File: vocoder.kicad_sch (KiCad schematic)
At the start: 66 parts, among them J1 AudioJack4, J2 Conn_01x02_Socket, J3 Conn_01x02_Pin, J4 USB_C_Receptacle_USB2.0_16P, Q1 Q_NPN_BCE, Q2 Q_NPN_BCE, Q3 AO3401A, Q4 Q_NPN_BCE, SW1 SW_SPDT, SW2 SW_Push, SW3 SW_Push, U2 MAX98357A, U3 BQ24074RGT, U4 TPS63031DSK, U5 ADAU1761, U6 ${SIM.PARAMS}, U7 ESP32-S3-WROOM-1

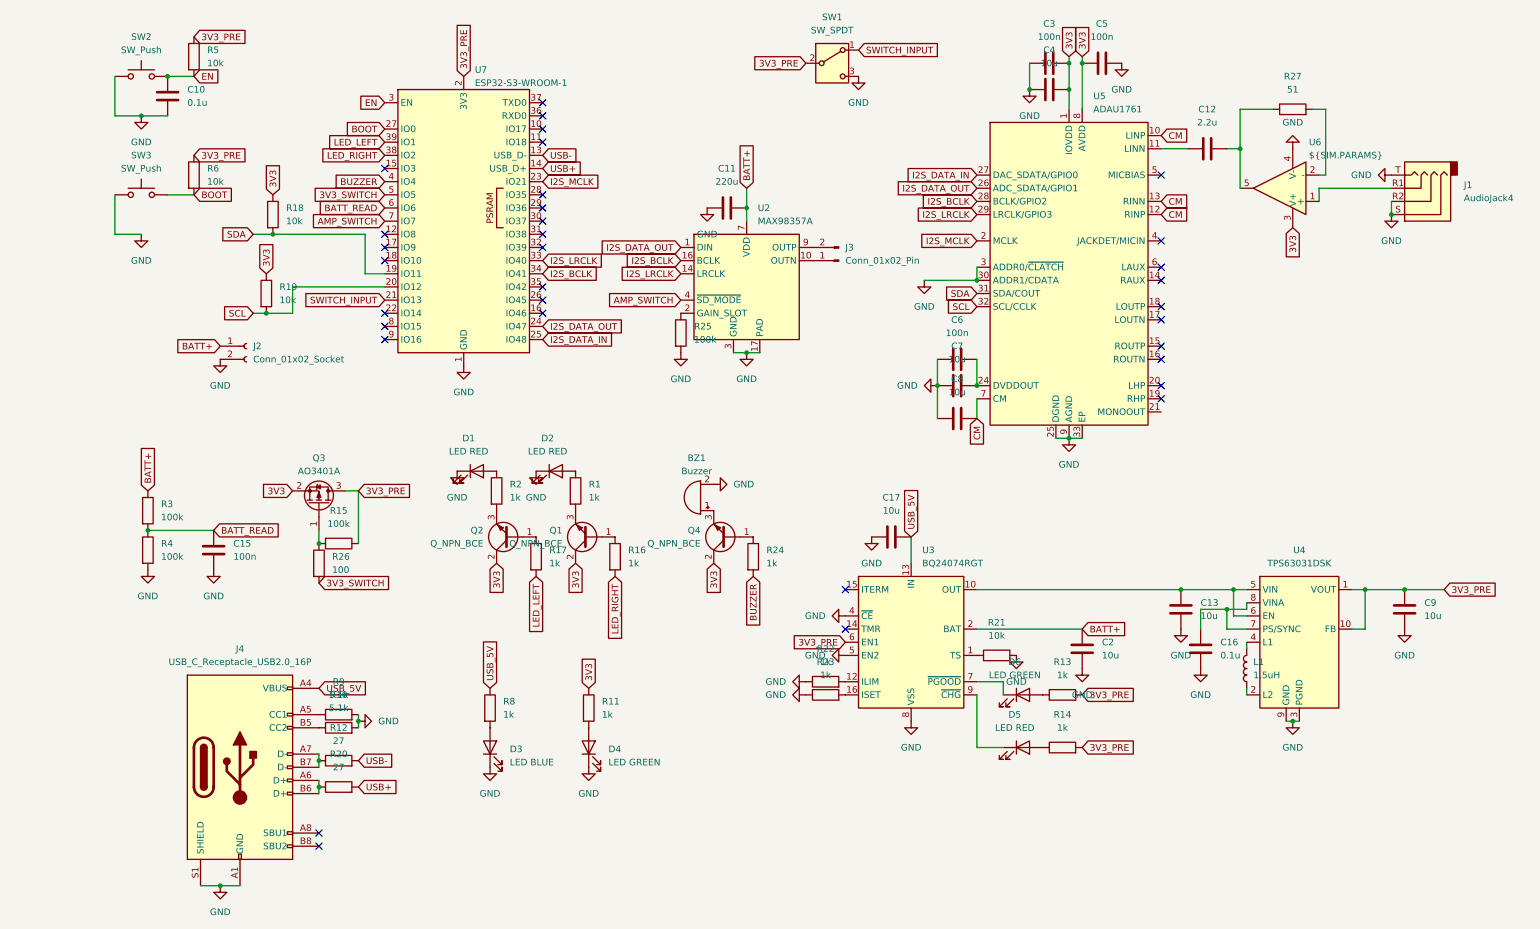
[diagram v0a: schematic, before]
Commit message: semi working before removing battery and adding necessary changes
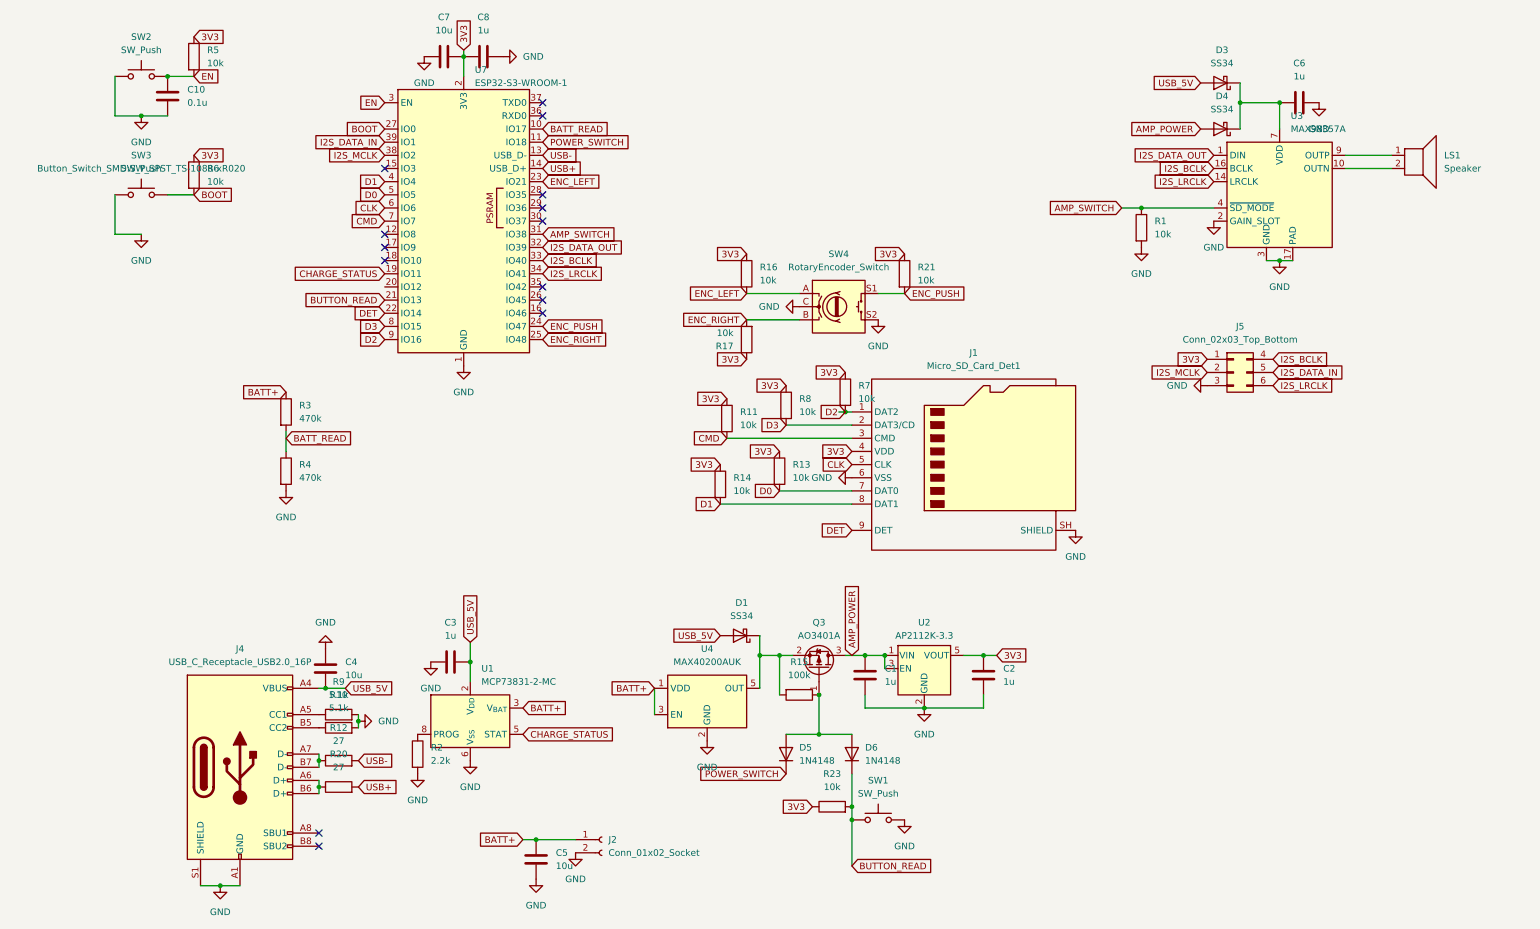
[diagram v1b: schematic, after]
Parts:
- removed BZ1: Buzzer, Connector_PinHeader_2.54mm:PinHeader_1x02_P2.54mm_Vertical, symbol Device:Buzzer
- removed C11: 220u, Capacitor_SMD:C_1206_3216Metric, symbol Device:C
- removed C12: 2.2u, Capacitor_SMD:C_0603_1608Metric, symbol Device:C
- removed C13, C17, C9: 10u, Capacitor_SMD:C_0603_1608Metric, symbol Device:C
- removed C15: 100n, Capacitor_SMD:C_0603_1608Metric, symbol Device:C
- removed C16: 0.1u, Capacitor_SMD:C_0603_1608Metric, symbol Device:C
- removed D1, D2, D5: LED RED, LED_SMD:LED_0603_1608Metric, symbol Device:LED
- removed D3: LED BLUE, LED_SMD:LED_0603_1608Metric, symbol Device:LED
- removed D4, D6: LED GREEN, LED_SMD:LED_0603_1608Metric, symbol Device:LED
- removed J1: AudioJack4, Connector_Audio:Jack_3.5mm_PJ320D_Horizontal, symbol Connector_Audio:AudioJack4
- removed J3: Conn_01x02_Pin, TerminalBlock_Phoenix:TerminalBlock_Phoenix_MKDS-1,5-2-5.08_1x02_P5.08mm_Horizontal, symbol Connector:Conn_01x02_Pin
- removed L1: 1.5uH, Inductor_SMD:L_0805_2012Metric, symbol Device:L
- removed Q1, Q2, Q4: Q_NPN_BCE, Package_TO_SOT_SMD:SOT-23, symbol Transistor_BJT:Q_NPN_BCE
- removed R18, R19: 10k, Resistor_SMD:R_0603_1608Metric_Pad0.98x0.95mm_HandSolder, symbol Device:R
- removed R22, R24: 1k, Resistor_SMD:R_0603_1608Metric_Pad0.98x0.95mm_HandSolder, symbol Device:R
- removed R25: 100k, Resistor_SMD:R_0603_1608Metric_Pad0.98x0.95mm_HandSolder, symbol Device:R
- removed R26: 100, Resistor_SMD:R_0603_1608Metric_Pad0.98x0.95mm_HandSolder, symbol Device:R
- removed R27: 51, Resistor_SMD:R_0603_1608Metric_Pad0.98x0.95mm_HandSolder, symbol Device:R
- removed SW1: SW_SPDT, Button_Switch_THT:SW_Slide-03_Wuerth-WS-SLTV_10x2.5x6.4_P2.54mm, symbol Switch:SW_SPDT
- removed U2: MAX98357A, Package_DFN_QFN:TQFN-16-1EP_3x3mm_P0.5mm_EP1.23x1.23mm, symbol Audio:MAX98357A
- removed U3: BQ24074RGT, Package_DFN_QFN:VQFN-16-1EP_3x3mm_P0.5mm_EP1.6x1.6mm, symbol Battery_Management:BQ24074RGT
- removed U4: TPS63031DSK, Package_SON:WSON-10-1EP_2.5x2.5mm_P0.5mm_EP1.2x2mm, symbol Regulator_Switching:TPS63031DSK
- removed U5: ADAU1761, Package_CSP:LFCSP-32-1EP_5x5mm_P0.5mm_EP3.5x3.5mm_ThermalVias, symbol Audio:ADAU1761
- removed U6: ${SIM.PARAMS}, custom_footprints:TLV9041, symbol Simulation_SPICE:OPAMP
- added C1: 1u, Capacitor_SMD:C_0603_1608Metric, symbol Device:C
- added D1, D3, D4: SS34, Diode_SMD:D_SOD-123, symbol Diode:SS34
- added D5, D6: 1N4148, Diode_SMD:D_SOD-323, symbol Diode:1N4148
- added J1: Micro_SD_Card_Det1, MyAntenna_manufacturer:Untitled, symbol Connector:Micro_SD_Card_Det1
- added J5: Conn_02x03_Top_Bottom, Connector_PinHeader_2.54mm:PinHeader_2x03_P2.54mm_Vertical, symbol Connector_Generic:Conn_02x03_Top_Bottom
- added LS1: Speaker, TerminalBlock_Phoenix:TerminalBlock_Phoenix_MKDS-1,5-2-5.08_1x02_P5.08mm_Horizontal, symbol Device:Speaker
- added R7: 10k, Resistor_SMD:R_0603_1608Metric_Pad0.98x0.95mm_HandSolder, symbol Device:R
- added SW1: SW_Push, Button_Switch_SMD:Panasonic_EVQPUJ_EVQPUA, symbol Switch:SW_Push
- added SW4: RotaryEncoder_Switch, Rotary_Encoder:RotaryEncoder_Bourns_Horizontal_PEC12R-2x17F-Sxxxx, symbol Device:RotaryEncoder_Switch
- added U1: MCP73831-2-MC, Package_DFN_QFN:DFN-8-1EP_3x2mm_P0.5mm_EP1.7x1.4mm, symbol Battery_Management:MCP73831-2-MC
- added U2: AP2112K-3.3, Package_TO_SOT_SMD:SOT-23-5, symbol Regulator_Linear:AP2112K-3.3
- added U3: MAX98357A, Package_DFN_QFN:TQFN-16-1EP_3x3mm_P0.5mm_EP1.23x1.23mm, symbol Audio:MAX98357A
- added U4: MAX40200AUK, Package_TO_SOT_SMD:SOT-23-5, symbol Analog_Switch:MAX40200AUK
- C2, C8: value 10u -> 1u
- C3, C6: value 100n -> 1u
- C4, C7: footprint Capacitor_SMD:C_0603_1608Metric -> Capacitor_SMD:C_0805_2012Metric
- C5: value 100n -> 10u; footprint Capacitor_SMD:C_0603_1608Metric -> Capacitor_SMD:C_0805_2012Metric
- R1, R11, R13, R14, R16, R17, R23, R8: value 1k -> 10k
- R2: value 1k -> 2.2k
- R3, R4: value 100k -> 470k
- SW2, SW3: footprint Button_Switch_SMD:SW_Push_SPST_NO_Alps_SKRK -> Button_Switch_SMD:SW_SPST_TS-1088-xR020
- U7: footprint RF_Module:ESP32-S3-WROOM-1 -> RF_Module:ESP32-S3-WROOM-1U
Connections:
- net CM is gone; now on net GND: C8.2
- net SWITCH_INPUT is gone; now on net BUTTON_READ: U7.21 (IO13)
- net 3V3: now also C2.1, C7.2, C8.1, R13.1, R14.1, R16.1, R17.1, R21.1, R23.1, R5.1, R6.1, R8.1, U7.2 (3V3), J1.4 (VDD), J5.1 (Pin_1), R7.1, U2.5 (VOUT); no longer C3.2, C4.2, C5.1, Q3.2 (S)
- net AMP_SWITCH: now also R1.1, U7.31 (IO38), U3.4 (~{SD_MODE}); no longer U7.7 (IO7)
- net BATT+: now also C5.2, U1.3 (V_{BAT}), U1.4 (V_{BAT}), U4.1 (VDD), U4.3 (EN); no longer C2.2
- net BATT_READ: now also U7.10 (IO17); no longer U7.6 (IO6)
- net GND: now also C2.2, C4.2, C5.1, C6.2, R1.2, R2.2, C1.2, J1.6 (VSS), J1.SH (SHIELD), J5.3 (Pin_3), SW1.2, SW4.C, SW4.S2, U1.6 (V_{SS}), U2.2 (GND), U3.11 (GND), U3.15 (GND), U3.17 (PAD), U3.2 (GAIN_SLOT), U3.3 (GND), U4.2 (GND); no longer C2.1, C4.1, C5.2, C6.1, C8.1, R21.2, R23.1
- net I2S_BCLK: now also U7.33 (IO40), J5.4 (Pin_4), U3.16 (BCLK); no longer U7.34 (IO41)
- net I2S_DATA_IN: now also U7.39 (IO1), J5.5 (Pin_5); no longer U7.25 (IO48)
- net I2S_DATA_OUT: now also U7.32 (IO39), U3.1 (DIN); no longer U7.24 (IO47)
- net I2S_LRCLK: now also U7.34 (IO41), J5.6 (Pin_6), U3.14 (LRCLK); no longer U7.33 (IO40)
- net I2S_MCLK: now also U7.38 (IO2), J5.2 (Pin_2); no longer U7.23 (IO21)
- net USB_5V: now also C3.2, C4.1, D1.2 (A), D3.2 (A), U1.1 (V_{DD}), U1.2 (V_{DD}); no longer R8.1
- net at Q3.1 (G): now also R15.1, D5.2 (A), D6.2 (A); no longer R15.2
- net BUTTON_READ: now reaches R23.2
- net BUTTON_READ: now also D6.1 (K), SW1.1
- net D3: now reaches R8.2
- net D3: now also U7.8 (IO15), J1.2 (DAT3/CD)
- net at R2.1: now also U1.8 (PROG)
- net CMD: now reaches R11.2
- net CMD: now also U7.7 (IO7), J1.3 (CMD)
- net POWER_SWITCH: now reaches U7.11 (IO18)
- net POWER_SWITCH: now also D5.1 (K)
- net DET: now reaches U7.22 (IO14)
- net DET: now also J1.9 (DET)
- net D2: now reaches U7.9 (IO16)
- net D2: now also J1.1 (DAT2), R7.2
- removed net 3V3_PRE: Q3.3 (D), R13.2, R14.2, R15.1, R5.1, R6.1, U7.2 (3V3)
- net 3V3_SWITCH renamed D0
- net D0: now also R13.2, J1.7 (DAT0)
- net BUZZER renamed D1
- net D1: now also R14.2, J1.8 (DAT1)
- net LED_LEFT renamed ENC_RIGHT
- net ENC_RIGHT: now also U7.25 (IO48), SW4.B; no longer U7.39 (IO1)
- net LED_RIGHT renamed ENC_LEFT
- net ENC_LEFT: now also U7.23 (IO21), SW4.A; no longer U7.38 (IO2)
- net SCL: no longer names the net of U7.20 (IO12)
- net SDA renamed CHARGE_STATUS
- net CHARGE_STATUS: now also U1.5 (STAT)
- new net: C6.1, D3.1 (K), D4.1 (K), U3.7 (VDD), U3.8 (VDD)
- new net: D1.1 (K), Q3.2 (S), R15.2, U4.5 (OUT)
- new net: LS1.1, U3.9 (OUTP)
- new net: LS1.2, U3.10 (OUTN)
- new net AMP_POWER: C1.1, D4.2 (A), Q3.3 (D), U2.1 (VIN), U2.3 (EN)
- new net CLK: J1.5 (CLK), U7.6 (IO6)
- new net ENC_PUSH: R21.2, SW4.S1, U7.24 (IO47)
- no-connect marks 33 -> 14
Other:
- moved on the sheet: J2, Q3, R15
